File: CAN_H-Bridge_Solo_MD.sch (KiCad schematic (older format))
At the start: 49 parts, among them IC1 SI8650AB-B-IS1, IC2 A3921KLPTR-T, IC3 AP7381-50SA-7, J2 Conn_01x03, J3 Conthrough, J4 Bus_mechaken_PCIexpress_x16_1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, M1 Motor_DC, Q1 IRFB3806PBF, Q2 IRFB3806PBF, Q3 IRFB3806PBF, Q4 IRFB3806PBF, U1 LDL1117S33R_SOT223-4, U2 STM32F042K6Tx, U3 MCP2562-E-SN, U4 LDL1117S33TR_SOT223-4

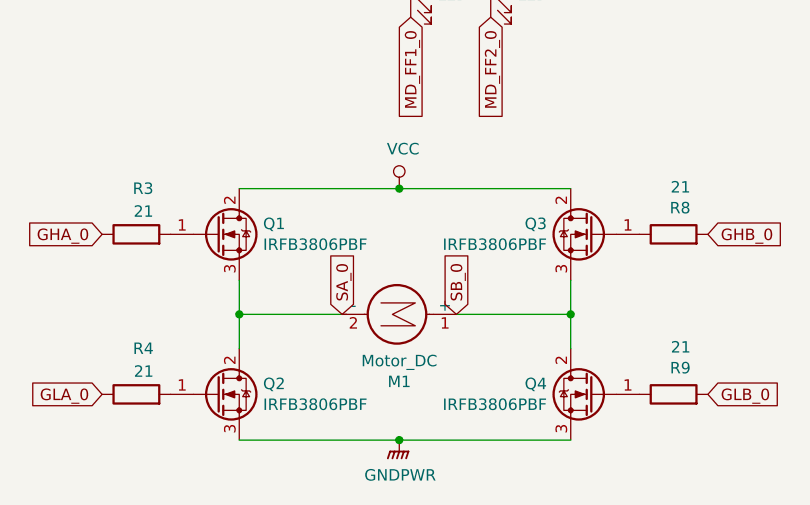
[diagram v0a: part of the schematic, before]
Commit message: fix
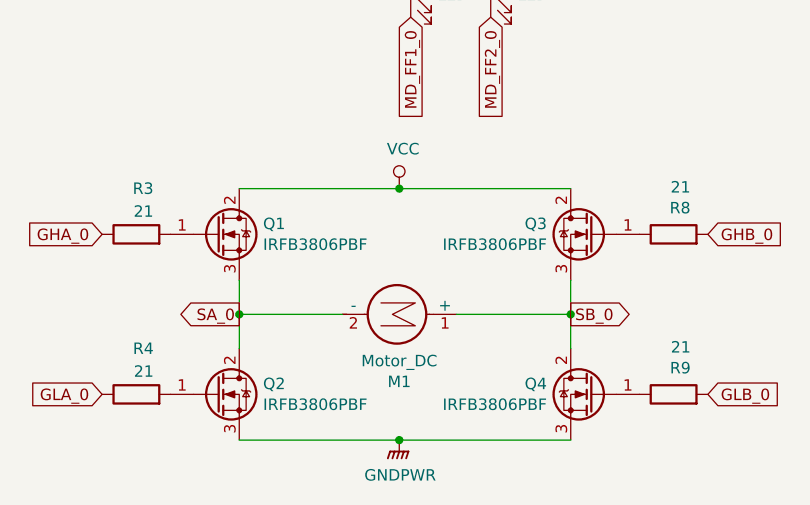
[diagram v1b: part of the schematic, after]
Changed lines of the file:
@@
 Wire Wire Line
 	2800 6700 2800 6850
-Text GLabel 3750 6700 1    50   Input ~ 0
+Text GLabel 4250 6700 2    50   Output ~ 0
 SB_0
-Text GLabel 3250 6700 1    50   Input ~ 0
-SA_0
 Wire Wire Line
 	7050 1600 7000 1600
@@
 NoConn ~ 3200 3000
 NoConn ~ 6800 1700
-$Comp
-L Motor:Motor_DC M1
-U 1 1 5E054D53
-P 3550 6700
-F 0 "M1" V 3845 6650 50  0000 C CNN
-F 1 "Motor_DC" V 3754 6650 50  0000 C CNN
-F 2 "XT60:XT60PW" H 3550 6610 50  0001 C CNN
-F 3 "~" H 3550 6610 50  0001 C CNN
-	1    3550 6700
-	0    1    1    0
-$EndComp
 Wire Wire Line
 	3750 6700 4250 6700
-Wire Wire Line
-	2800 6700 3250 6700
 Text GLabel 10700 5250 2    50   Input ~ 0
 V5
@@
 Wire Wire Line
 	1700 1700 1700 1950
+Wire Wire Line
+	2800 6700 3250 6700
+$Comp
+L Motor:Motor_DC M1
+U 1 1 5E054D53
+P 3550 6700
+F 0 "M1" V 3845 6650 50  0000 C CNN
+F 1 "Motor_DC" V 3754 6650 50  0000 C CNN
+F 2 "XT60:XT60PW" H 3550 6610 50  0001 C CNN
+F 3 "~" H 3550 6610 50  0001 C CNN
+	1    3550 6700
+	0    1    1    0
+$EndComp
+Text GLabel 2800 6700 0    50   Output ~ 0
+SA_0
 $EndSCHEMATC
